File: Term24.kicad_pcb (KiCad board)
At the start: 4 copper layers, 100 x 60 mm, 55 parts, among them J1 USB_B, J11 VGA DE15, J14 Conn_01x06, J15 Conn_01x06, J3 DE9_Plug, J5 Mini-DIN-6, J6 Conn_01x08, J7 AudioJack3, SW1 SW_DIP_x02, SW11 SW_Push, SW2 SW_DIP_x02, SW3 SW_SPDT, U1 PIC24EP512GP202-I/SP, U5 LM1117T-3.3

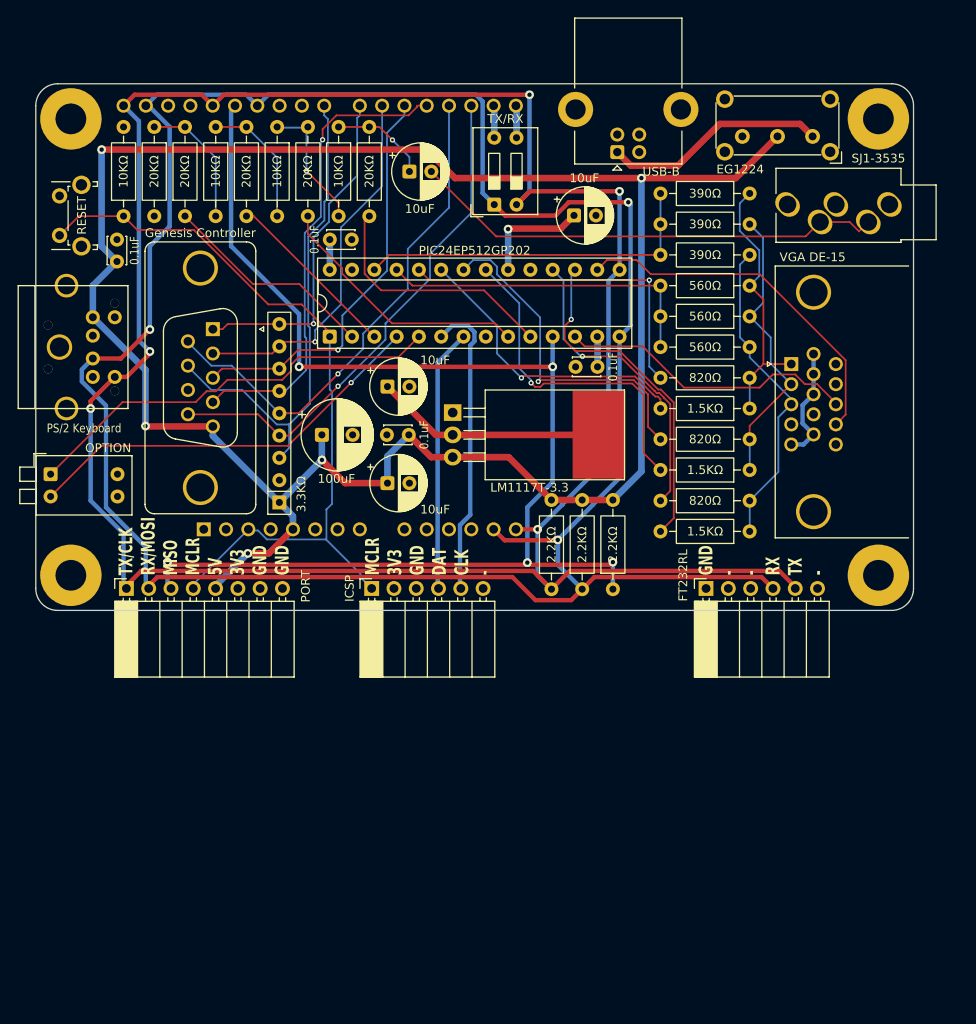
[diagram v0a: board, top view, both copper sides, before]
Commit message: Add files via upload
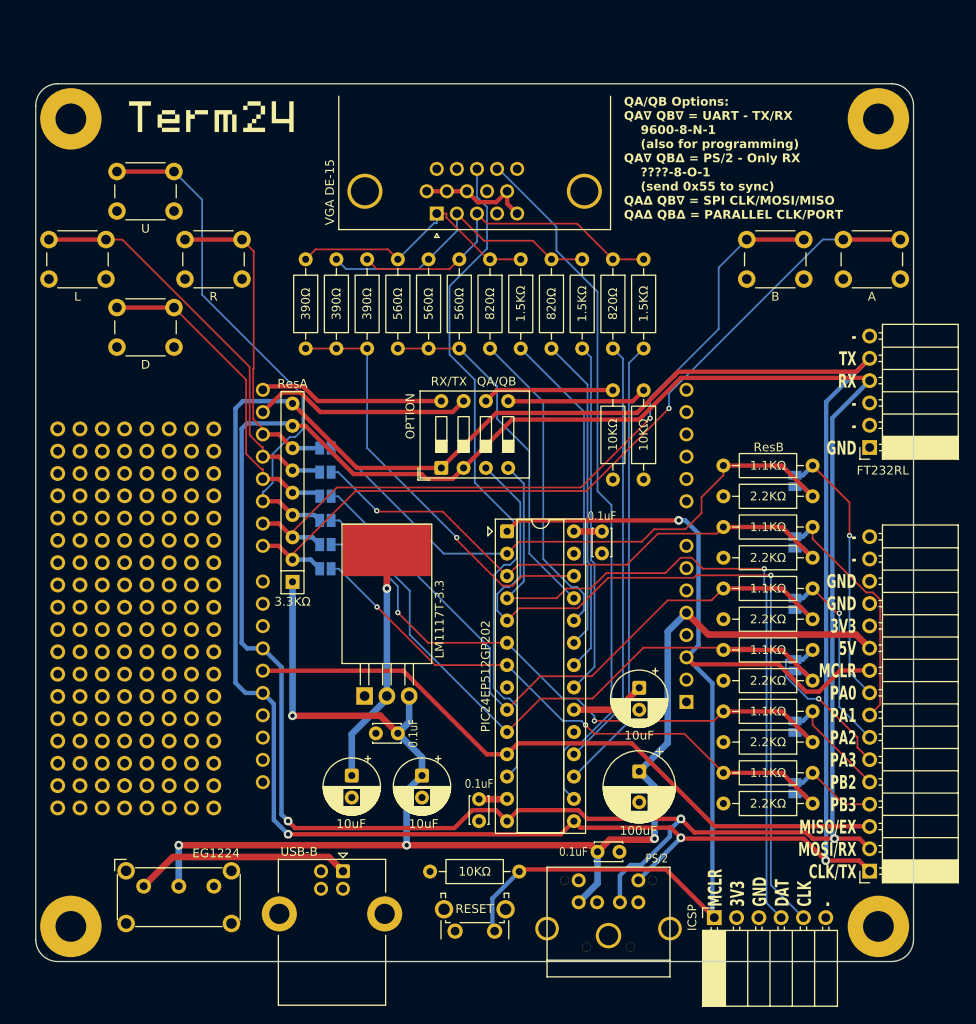
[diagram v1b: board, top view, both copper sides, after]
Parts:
- removed C24: C_Polarized_Small_US, Capacitor_THT:CP_Radial_D6.3mm_P2.50mm
- removed J3: DE9_Plug, Connector_Dsub:DSUB-9_Pins_Vertical_P2.77x2.84mm_MountingHoles
- removed J6: Conn_01x08, Connector_PinSocket_2.54mm:PinSocket_1x08_P2.54mm_Horizontal
- removed J7: AudioJack3, Connector_Audio:Jack_3.5mm_CUI_SJ1-3535NG_Horizontal_CircularHoles
- removed R21, R22, R23, R24, R25, R26, R27, R4, R5, R6: R_US, Resistor_THT:R_Axial_DIN0207_L6.3mm_D2.5mm_P10.16mm_Horizontal
- removed SW1: SW_DIP_x02, Button_Switch_THT:SW_DIP_SPSTx02_Slide_9.78x7.26mm_W7.62mm_P2.54mm
- removed SW2: SW_DIP_x02, Button_Switch_THT:SW_DIP_SPSTx02_Piano_10.8x6.64mm_W7.62mm_P2.54mm
- added J2: Conn_01x16, Connector_PinSocket_2.54mm:PinSocket_1x16_P2.54mm_Horizontal, F.Cu at (145.0, 139.7)
- added JP1: Jumper_2_Open, Jumper:SolderJumper-2_P1.3mm_Open_Pad1.0x1.5mm, B.Cu at (136.5, 95.2)
- added JP10: Jumper_2_Open, Jumper:SolderJumper-2_P1.3mm_Open_Pad1.0x1.5mm, B.Cu at (83.0, 99.8)
- added JP11: Jumper_2_Open, Jumper:SolderJumper-2_P1.3mm_Open_Pad1.0x1.5mm, B.Cu at (83.0, 102.5)
- added JP12: Jumper_2_Open, Jumper:SolderJumper-2_P1.3mm_Open_Pad1.0x1.5mm, B.Cu at (83.0, 105.2)
- added JP2: Jumper_2_Open, Jumper:SolderJumper-2_P1.3mm_Open_Pad1.0x1.5mm, B.Cu at (136.5, 102.2)
- added JP3: Jumper_2_Open, Jumper:SolderJumper-2_P1.3mm_Open_Pad1.0x1.5mm, B.Cu at (136.5, 109.2)
- added JP4: Jumper_2_Open, Jumper:SolderJumper-2_P1.3mm_Open_Pad1.0x1.5mm, B.Cu at (136.5, 116.2)
- added JP5: Jumper_2_Open, Jumper:SolderJumper-2_P1.3mm_Open_Pad1.0x1.5mm, B.Cu at (136.5, 123.2)
- added JP6: Jumper_2_Open, Jumper:SolderJumper-2_P1.3mm_Open_Pad1.0x1.5mm, B.Cu at (136.5, 130.2)
- added JP7: Jumper_2_Open, Jumper:SolderJumper-2_P1.3mm_Open_Pad1.0x1.5mm, B.Cu at (83.0, 91.5)
- added JP8: Jumper_2_Open, Jumper:SolderJumper-2_P1.3mm_Open_Pad1.0x1.5mm, B.Cu at (83.0, 94.2)
- added JP9: Jumper_2_Open, Jumper:SolderJumper-2_P1.3mm_Open_Pad1.0x1.5mm, B.Cu at (83.0, 97.0)
- added R33: R_US, Resistor_THT:R_Axial_DIN0207_L6.3mm_D2.5mm_P10.16mm_Horizontal, F.Cu at (115.8, 95.1)
- added R34: R_US, Resistor_THT:R_Axial_DIN0207_L6.3mm_D2.5mm_P10.16mm_Horizontal, F.Cu at (119.2, 95.1)
- added R35: R_US, Resistor_THT:R_Axial_DIN0207_L6.3mm_D2.5mm_P10.16mm_Horizontal, F.Cu at (138.5, 93.5)
- added R37: R_US, Resistor_THT:R_Axial_DIN0207_L6.3mm_D2.5mm_P10.16mm_Horizontal, F.Cu at (138.5, 100.5)
- added R38: R_US, Resistor_THT:R_Axial_DIN0207_L6.3mm_D2.5mm_P10.16mm_Horizontal, F.Cu at (138.5, 104.0)
- added R39: R_US, Resistor_THT:R_Axial_DIN0207_L6.3mm_D2.5mm_P10.16mm_Horizontal, F.Cu at (138.5, 107.5)
- added R40: R_US, Resistor_THT:R_Axial_DIN0207_L6.3mm_D2.5mm_P10.16mm_Horizontal, F.Cu at (138.5, 111.0)
- added R41: R_US, Resistor_THT:R_Axial_DIN0207_L6.3mm_D2.5mm_P10.16mm_Horizontal, F.Cu at (138.5, 114.5)
- added R42: R_US, Resistor_THT:R_Axial_DIN0207_L6.3mm_D2.5mm_P10.16mm_Horizontal, F.Cu at (138.5, 118.0)
- added R43: R_US, Resistor_THT:R_Axial_DIN0207_L6.3mm_D2.5mm_P10.16mm_Horizontal, F.Cu at (138.5, 121.5)
- added R44: R_US, Resistor_THT:R_Axial_DIN0207_L6.3mm_D2.5mm_P10.16mm_Horizontal, F.Cu at (138.5, 125.0)
- added R45: R_US, Resistor_THT:R_Axial_DIN0207_L6.3mm_D2.5mm_P10.16mm_Horizontal, F.Cu at (138.5, 128.5)
- added R46: R_US, Resistor_THT:R_Axial_DIN0207_L6.3mm_D2.5mm_P10.16mm_Horizontal, F.Cu at (138.5, 132.0)
- added SW10: SW_DIP_x04, Button_Switch_THT:SW_DIP_SPSTx04_Slide_9.78x12.34mm_W7.62mm_P2.54mm, F.Cu at (96.2, 93.8)
- added SW4: SW_Push, Button_Switch_THT:SW_PUSH_6mm_H7.3mm, F.Cu at (59.2, 60.0)
- added SW5: SW_Push, Button_Switch_THT:SW_PUSH_6mm_H7.3mm, F.Cu at (59.2, 75.5)
- added SW6: SW_Push, Button_Switch_THT:SW_PUSH_6mm_H7.3mm, F.Cu at (51.5, 67.8)
- added SW7: SW_Push, Button_Switch_THT:SW_PUSH_6mm_H7.3mm, F.Cu at (67.0, 67.8)
- added SW8: SW_Push, Button_Switch_THT:SW_PUSH_6mm_H7.3mm, F.Cu at (142.0, 67.8)
- added SW9: SW_Push, Button_Switch_THT:SW_PUSH_6mm_H7.3mm, F.Cu at (131.0, 67.8)
- added TP1: TestPoint, Hardware:PinHeader_1x01_P2.54mm_Vertical_TestPoint, F.Cu at (52.5, 89.3)
- added TP10: TestPoint, Hardware:PinHeader_1x01_P2.54mm_Vertical_TestPoint, F.Cu at (67.7, 89.3)
- added TP100: TestPoint, Hardware:PinHeader_1x01_P2.54mm_Vertical_TestPoint, F.Cu at (70.3, 117.3)
- added TP101: TestPoint, Hardware:PinHeader_1x01_P2.54mm_Vertical_TestPoint, F.Cu at (52.5, 119.8)
- added TP102: TestPoint, Hardware:PinHeader_1x01_P2.54mm_Vertical_TestPoint, F.Cu at (52.5, 122.3)
- added TP103: TestPoint, Hardware:PinHeader_1x01_P2.54mm_Vertical_TestPoint, F.Cu at (52.5, 124.9)
- added TP104: TestPoint, Hardware:PinHeader_1x01_P2.54mm_Vertical_TestPoint, F.Cu at (52.5, 127.4)
- added TP105: TestPoint, Hardware:PinHeader_1x01_P2.54mm_Vertical_TestPoint, F.Cu at (52.5, 130.0)
- added TP106: TestPoint, Hardware:PinHeader_1x01_P2.54mm_Vertical_TestPoint, F.Cu at (52.5, 132.5)
- added TP107: TestPoint, Hardware:PinHeader_1x01_P2.54mm_Vertical_TestPoint, F.Cu at (55.0, 119.8)
- added TP108: TestPoint, Hardware:PinHeader_1x01_P2.54mm_Vertical_TestPoint, F.Cu at (55.0, 122.3)
- added TP109: TestPoint, Hardware:PinHeader_1x01_P2.54mm_Vertical_TestPoint, F.Cu at (55.0, 124.9)
- added TP11: TestPoint, Hardware:PinHeader_1x01_P2.54mm_Vertical_TestPoint, F.Cu at (60.1, 89.3)
- added TP110: TestPoint, Hardware:PinHeader_1x01_P2.54mm_Vertical_TestPoint, F.Cu at (55.0, 127.4)
- added TP111: TestPoint, Hardware:PinHeader_1x01_P2.54mm_Vertical_TestPoint, F.Cu at (55.0, 130.0)
- added TP112: TestPoint, Hardware:PinHeader_1x01_P2.54mm_Vertical_TestPoint, F.Cu at (55.0, 132.5)
- added TP113: TestPoint, Hardware:PinHeader_1x01_P2.54mm_Vertical_TestPoint, F.Cu at (57.6, 119.8)
- added TP114: TestPoint, Hardware:PinHeader_1x01_P2.54mm_Vertical_TestPoint, F.Cu at (57.6, 122.3)
- added TP115: TestPoint, Hardware:PinHeader_1x01_P2.54mm_Vertical_TestPoint, F.Cu at (57.6, 124.9)
- added TP116: TestPoint, Hardware:PinHeader_1x01_P2.54mm_Vertical_TestPoint, F.Cu at (57.6, 127.4)
- added TP117: TestPoint, Hardware:PinHeader_1x01_P2.54mm_Vertical_TestPoint, F.Cu at (57.6, 130.0)
- added TP118: TestPoint, Hardware:PinHeader_1x01_P2.54mm_Vertical_TestPoint, F.Cu at (57.6, 132.5)
- added TP119: TestPoint, Hardware:PinHeader_1x01_P2.54mm_Vertical_TestPoint, F.Cu at (60.1, 119.8)
- added TP12: TestPoint, Hardware:PinHeader_1x01_P2.54mm_Vertical_TestPoint, F.Cu at (70.3, 89.3)
- added TP120: TestPoint, Hardware:PinHeader_1x01_P2.54mm_Vertical_TestPoint, F.Cu at (60.1, 122.3)
- added TP121: TestPoint, Hardware:PinHeader_1x01_P2.54mm_Vertical_TestPoint, F.Cu at (60.1, 124.9)
- added TP122: TestPoint, Hardware:PinHeader_1x01_P2.54mm_Vertical_TestPoint, F.Cu at (60.1, 127.4)
- added TP123: TestPoint, Hardware:PinHeader_1x01_P2.54mm_Vertical_TestPoint, F.Cu at (60.1, 130.0)
- added TP124: TestPoint, Hardware:PinHeader_1x01_P2.54mm_Vertical_TestPoint, F.Cu at (60.1, 132.5)
- added TP125: TestPoint, Hardware:PinHeader_1x01_P2.54mm_Vertical_TestPoint, F.Cu at (62.7, 119.8)
- added TP126: TestPoint, Hardware:PinHeader_1x01_P2.54mm_Vertical_TestPoint, F.Cu at (62.7, 122.3)
- added TP127: TestPoint, Hardware:PinHeader_1x01_P2.54mm_Vertical_TestPoint, F.Cu at (62.7, 124.9)
- added TP128: TestPoint, Hardware:PinHeader_1x01_P2.54mm_Vertical_TestPoint, F.Cu at (62.7, 127.4)
- added TP129: TestPoint, Hardware:PinHeader_1x01_P2.54mm_Vertical_TestPoint, F.Cu at (62.7, 130.0)
- added TP13: TestPoint, Hardware:PinHeader_1x01_P2.54mm_Vertical_TestPoint, F.Cu at (52.5, 91.9)
- added TP130: TestPoint, Hardware:PinHeader_1x01_P2.54mm_Vertical_TestPoint, F.Cu at (62.7, 132.5)
- added TP131: TestPoint, Hardware:PinHeader_1x01_P2.54mm_Vertical_TestPoint, F.Cu at (65.2, 119.8)
- added TP132: TestPoint, Hardware:PinHeader_1x01_P2.54mm_Vertical_TestPoint, F.Cu at (65.2, 122.3)
- added TP133: TestPoint, Hardware:PinHeader_1x01_P2.54mm_Vertical_TestPoint, F.Cu at (65.2, 124.9)
- added TP134: TestPoint, Hardware:PinHeader_1x01_P2.54mm_Vertical_TestPoint, F.Cu at (65.2, 127.4)
- added TP135: TestPoint, Hardware:PinHeader_1x01_P2.54mm_Vertical_TestPoint, F.Cu at (65.2, 130.0)
- added TP136: TestPoint, Hardware:PinHeader_1x01_P2.54mm_Vertical_TestPoint, F.Cu at (65.2, 132.5)
- added TP137: TestPoint, Hardware:PinHeader_1x01_P2.54mm_Vertical_TestPoint, F.Cu at (67.7, 119.8)
- added TP138: TestPoint, Hardware:PinHeader_1x01_P2.54mm_Vertical_TestPoint, F.Cu at (67.7, 122.3)
- added TP139: TestPoint, Hardware:PinHeader_1x01_P2.54mm_Vertical_TestPoint, F.Cu at (67.7, 124.9)
- added TP14: TestPoint, Hardware:PinHeader_1x01_P2.54mm_Vertical_TestPoint, F.Cu at (55.0, 91.9)
- added TP140: TestPoint, Hardware:PinHeader_1x01_P2.54mm_Vertical_TestPoint, F.Cu at (67.7, 127.4)
- added TP141: TestPoint, Hardware:PinHeader_1x01_P2.54mm_Vertical_TestPoint, F.Cu at (67.7, 130.0)
- added TP142: TestPoint, Hardware:PinHeader_1x01_P2.54mm_Vertical_TestPoint, F.Cu at (67.7, 132.5)
- added TP143: TestPoint, Hardware:PinHeader_1x01_P2.54mm_Vertical_TestPoint, F.Cu at (70.3, 119.8)
- added TP144: TestPoint, Hardware:PinHeader_1x01_P2.54mm_Vertical_TestPoint, F.Cu at (70.3, 122.3)
- added TP145: TestPoint, Hardware:PinHeader_1x01_P2.54mm_Vertical_TestPoint, F.Cu at (70.3, 124.9)
- added TP146: TestPoint, Hardware:PinHeader_1x01_P2.54mm_Vertical_TestPoint, F.Cu at (70.3, 127.4)
- added TP147: TestPoint, Hardware:PinHeader_1x01_P2.54mm_Vertical_TestPoint, F.Cu at (70.3, 130.0)
- added TP148: TestPoint, Hardware:PinHeader_1x01_P2.54mm_Vertical_TestPoint, F.Cu at (70.3, 132.5)
- added TP15: TestPoint, Hardware:PinHeader_1x01_P2.54mm_Vertical_TestPoint, F.Cu at (55.0, 94.4)
- added TP16: TestPoint, Hardware:PinHeader_1x01_P2.54mm_Vertical_TestPoint, F.Cu at (52.5, 99.5)
- added TP17: TestPoint, Hardware:PinHeader_1x01_P2.54mm_Vertical_TestPoint, F.Cu at (52.5, 102.0)
- added TP18: TestPoint, Hardware:PinHeader_1x01_P2.54mm_Vertical_TestPoint, F.Cu at (52.5, 104.6)
- added TP19: TestPoint, Hardware:PinHeader_1x01_P2.54mm_Vertical_TestPoint, F.Cu at (52.5, 107.1)
- added TP20: TestPoint, Hardware:PinHeader_1x01_P2.54mm_Vertical_TestPoint, F.Cu at (52.5, 109.6)
- added TP21: TestPoint, Hardware:PinHeader_1x01_P2.54mm_Vertical_TestPoint, F.Cu at (52.5, 112.2)
- added TP22: TestPoint, Hardware:PinHeader_1x01_P2.54mm_Vertical_TestPoint, F.Cu at (52.5, 114.7)
- added TP23: TestPoint, Hardware:PinHeader_1x01_P2.54mm_Vertical_TestPoint, F.Cu at (52.5, 117.3)
- added TP24: TestPoint, Hardware:PinHeader_1x01_P2.54mm_Vertical_TestPoint, F.Cu at (57.6, 91.9)
- added TP25: TestPoint, Hardware:PinHeader_1x01_P2.54mm_Vertical_TestPoint, F.Cu at (52.5, 94.4)
- added TP26: TestPoint, Hardware:PinHeader_1x01_P2.54mm_Vertical_TestPoint, F.Cu at (57.6, 94.4)
- added TP27: TestPoint, Hardware:PinHeader_1x01_P2.54mm_Vertical_TestPoint, F.Cu at (55.0, 99.5)
- added TP28: TestPoint, Hardware:PinHeader_1x01_P2.54mm_Vertical_TestPoint, F.Cu at (55.0, 102.0)
- added TP29: TestPoint, Hardware:PinHeader_1x01_P2.54mm_Vertical_TestPoint, F.Cu at (55.0, 104.6)
- added TP30: TestPoint, Hardware:PinHeader_1x01_P2.54mm_Vertical_TestPoint, F.Cu at (55.0, 107.1)
- added TP31: TestPoint, Hardware:PinHeader_1x01_P2.54mm_Vertical_TestPoint, F.Cu at (55.0, 109.6)
- added TP32: TestPoint, Hardware:PinHeader_1x01_P2.54mm_Vertical_TestPoint, F.Cu at (55.0, 112.2)
- added TP33: TestPoint, Hardware:PinHeader_1x01_P2.54mm_Vertical_TestPoint, F.Cu at (55.0, 114.7)
- added TP34: TestPoint, Hardware:PinHeader_1x01_P2.54mm_Vertical_TestPoint, F.Cu at (55.0, 117.3)
- added TP35: TestPoint, Hardware:PinHeader_1x01_P2.54mm_Vertical_TestPoint, F.Cu at (60.1, 91.9)
- added TP36: TestPoint, Hardware:PinHeader_1x01_P2.54mm_Vertical_TestPoint, F.Cu at (60.1, 94.4)
- added TP37: TestPoint, Hardware:PinHeader_1x01_P2.54mm_Vertical_TestPoint, F.Cu at (52.5, 96.9)
- added TP38: TestPoint, Hardware:PinHeader_1x01_P2.54mm_Vertical_TestPoint, F.Cu at (57.6, 99.5)
- added TP39: TestPoint, Hardware:PinHeader_1x01_P2.54mm_Vertical_TestPoint, F.Cu at (57.6, 102.0)
- added TP40: TestPoint, Hardware:PinHeader_1x01_P2.54mm_Vertical_TestPoint, F.Cu at (57.6, 104.6)
- added TP41: TestPoint, Hardware:PinHeader_1x01_P2.54mm_Vertical_TestPoint, F.Cu at (57.6, 107.1)
- added TP42: TestPoint, Hardware:PinHeader_1x01_P2.54mm_Vertical_TestPoint, F.Cu at (57.6, 109.6)
- added TP43: TestPoint, Hardware:PinHeader_1x01_P2.54mm_Vertical_TestPoint, F.Cu at (57.6, 112.2)
- added TP44: TestPoint, Hardware:PinHeader_1x01_P2.54mm_Vertical_TestPoint, F.Cu at (57.6, 114.7)
- added TP45: TestPoint, Hardware:PinHeader_1x01_P2.54mm_Vertical_TestPoint, F.Cu at (57.6, 117.3)
- added TP46: TestPoint, Hardware:PinHeader_1x01_P2.54mm_Vertical_TestPoint, F.Cu at (62.7, 91.9)
- added TP47: TestPoint, Hardware:PinHeader_1x01_P2.54mm_Vertical_TestPoint, F.Cu at (62.7, 94.4)
- added TP48: TestPoint, Hardware:PinHeader_1x01_P2.54mm_Vertical_TestPoint, F.Cu at (55.0, 96.9)
- added TP49: TestPoint, Hardware:PinHeader_1x01_P2.54mm_Vertical_TestPoint, F.Cu at (60.1, 99.5)
- added TP50: TestPoint, Hardware:PinHeader_1x01_P2.54mm_Vertical_TestPoint, F.Cu at (60.1, 102.0)
- added TP51: TestPoint, Hardware:PinHeader_1x01_P2.54mm_Vertical_TestPoint, F.Cu at (60.1, 104.6)
- added TP52: TestPoint, Hardware:PinHeader_1x01_P2.54mm_Vertical_TestPoint, F.Cu at (60.1, 107.1)
- added TP53: TestPoint, Hardware:PinHeader_1x01_P2.54mm_Vertical_TestPoint, F.Cu at (60.1, 109.6)
- added TP54: TestPoint, Hardware:PinHeader_1x01_P2.54mm_Vertical_TestPoint, F.Cu at (60.1, 112.2)
- added TP55: TestPoint, Hardware:PinHeader_1x01_P2.54mm_Vertical_TestPoint, F.Cu at (60.1, 114.7)
- added TP56: TestPoint, Hardware:PinHeader_1x01_P2.54mm_Vertical_TestPoint, F.Cu at (60.1, 117.3)
- added TP57: TestPoint, Hardware:PinHeader_1x01_P2.54mm_Vertical_TestPoint, F.Cu at (65.2, 91.9)
- added TP58: TestPoint, Hardware:PinHeader_1x01_P2.54mm_Vertical_TestPoint, F.Cu at (65.2, 94.4)
- added TP59: TestPoint, Hardware:PinHeader_1x01_P2.54mm_Vertical_TestPoint, F.Cu at (57.6, 96.9)
- added TP6: TestPoint, Hardware:PinHeader_1x01_P2.54mm_Vertical_TestPoint, F.Cu at (62.7, 89.3)
- added TP60: TestPoint, Hardware:PinHeader_1x01_P2.54mm_Vertical_TestPoint, F.Cu at (62.7, 99.5)
- added TP61: TestPoint, Hardware:PinHeader_1x01_P2.54mm_Vertical_TestPoint, F.Cu at (62.7, 102.0)
- added TP62: TestPoint, Hardware:PinHeader_1x01_P2.54mm_Vertical_TestPoint, F.Cu at (62.7, 104.6)
- added TP63: TestPoint, Hardware:PinHeader_1x01_P2.54mm_Vertical_TestPoint, F.Cu at (62.7, 107.1)
- added TP64: TestPoint, Hardware:PinHeader_1x01_P2.54mm_Vertical_TestPoint, F.Cu at (62.7, 109.6)
- added TP65: TestPoint, Hardware:PinHeader_1x01_P2.54mm_Vertical_TestPoint, F.Cu at (62.7, 112.2)
- added TP66: TestPoint, Hardware:PinHeader_1x01_P2.54mm_Vertical_TestPoint, F.Cu at (62.7, 114.7)
- added TP67: TestPoint, Hardware:PinHeader_1x01_P2.54mm_Vertical_TestPoint, F.Cu at (62.7, 117.3)
- added TP68: TestPoint, Hardware:PinHeader_1x01_P2.54mm_Vertical_TestPoint, F.Cu at (67.7, 91.9)
- added TP69: TestPoint, Hardware:PinHeader_1x01_P2.54mm_Vertical_TestPoint, F.Cu at (67.7, 94.4)
- added TP7: TestPoint, Hardware:PinHeader_1x01_P2.54mm_Vertical_TestPoint, F.Cu at (55.0, 89.3)
- added TP70: TestPoint, Hardware:PinHeader_1x01_P2.54mm_Vertical_TestPoint, F.Cu at (60.1, 96.9)
- added TP71: TestPoint, Hardware:PinHeader_1x01_P2.54mm_Vertical_TestPoint, F.Cu at (65.2, 99.5)
- added TP72: TestPoint, Hardware:PinHeader_1x01_P2.54mm_Vertical_TestPoint, F.Cu at (65.2, 102.0)
- added TP73: TestPoint, Hardware:PinHeader_1x01_P2.54mm_Vertical_TestPoint, F.Cu at (65.2, 104.6)
- added TP74: TestPoint, Hardware:PinHeader_1x01_P2.54mm_Vertical_TestPoint, F.Cu at (65.2, 107.1)
- added TP75: TestPoint, Hardware:PinHeader_1x01_P2.54mm_Vertical_TestPoint, F.Cu at (65.2, 109.6)
- added TP76: TestPoint, Hardware:PinHeader_1x01_P2.54mm_Vertical_TestPoint, F.Cu at (65.2, 112.2)
- added TP77: TestPoint, Hardware:PinHeader_1x01_P2.54mm_Vertical_TestPoint, F.Cu at (65.2, 114.7)
- added TP78: TestPoint, Hardware:PinHeader_1x01_P2.54mm_Vertical_TestPoint, F.Cu at (65.2, 117.3)
- added TP79: TestPoint, Hardware:PinHeader_1x01_P2.54mm_Vertical_TestPoint, F.Cu at (70.3, 91.9)
- added TP8: TestPoint, Hardware:PinHeader_1x01_P2.54mm_Vertical_TestPoint, F.Cu at (65.2, 89.3)
- added TP80: TestPoint, Hardware:PinHeader_1x01_P2.54mm_Vertical_TestPoint, F.Cu at (67.7, 96.9)
- added TP81: TestPoint, Hardware:PinHeader_1x01_P2.54mm_Vertical_TestPoint, F.Cu at (62.7, 96.9)
- added TP82: TestPoint, Hardware:PinHeader_1x01_P2.54mm_Vertical_TestPoint, F.Cu at (67.7, 99.5)
- added TP83: TestPoint, Hardware:PinHeader_1x01_P2.54mm_Vertical_TestPoint, F.Cu at (67.7, 102.0)
- added TP84: TestPoint, Hardware:PinHeader_1x01_P2.54mm_Vertical_TestPoint, F.Cu at (67.7, 104.6)
- added TP85: TestPoint, Hardware:PinHeader_1x01_P2.54mm_Vertical_TestPoint, F.Cu at (67.7, 107.1)
- added TP86: TestPoint, Hardware:PinHeader_1x01_P2.54mm_Vertical_TestPoint, F.Cu at (67.7, 109.6)
- added TP87: TestPoint, Hardware:PinHeader_1x01_P2.54mm_Vertical_TestPoint, F.Cu at (67.7, 112.2)
- added TP88: TestPoint, Hardware:PinHeader_1x01_P2.54mm_Vertical_TestPoint, F.Cu at (67.7, 114.7)
- added TP89: TestPoint, Hardware:PinHeader_1x01_P2.54mm_Vertical_TestPoint, F.Cu at (67.7, 117.3)
- added TP9: TestPoint, Hardware:PinHeader_1x01_P2.54mm_Vertical_TestPoint, F.Cu at (57.6, 89.3)
- added TP90: TestPoint, Hardware:PinHeader_1x01_P2.54mm_Vertical_TestPoint, F.Cu at (70.3, 94.4)
- added TP91: TestPoint, Hardware:PinHeader_1x01_P2.54mm_Vertical_TestPoint, F.Cu at (70.3, 96.9)
- added TP92: TestPoint, Hardware:PinHeader_1x01_P2.54mm_Vertical_TestPoint, F.Cu at (65.2, 96.9)
- added TP93: TestPoint, Hardware:PinHeader_1x01_P2.54mm_Vertical_TestPoint, F.Cu at (70.3, 99.5)
- added TP94: TestPoint, Hardware:PinHeader_1x01_P2.54mm_Vertical_TestPoint, F.Cu at (70.3, 102.0)
- added TP95: TestPoint, Hardware:PinHeader_1x01_P2.54mm_Vertical_TestPoint, F.Cu at (70.3, 104.6)
- added TP96: TestPoint, Hardware:PinHeader_1x01_P2.54mm_Vertical_TestPoint, F.Cu at (70.3, 107.1)
- added TP97: TestPoint, Hardware:PinHeader_1x01_P2.54mm_Vertical_TestPoint, F.Cu at (70.3, 109.6)
- added TP98: TestPoint, Hardware:PinHeader_1x01_P2.54mm_Vertical_TestPoint, F.Cu at (70.3, 112.2)
- added TP99: TestPoint, Hardware:PinHeader_1x01_P2.54mm_Vertical_TestPoint, F.Cu at (70.3, 114.7)
- G102: moved to F.Cu
- moved SW3 114.5 mm to (62.3, 141.4), turned to 0 degrees
- moved SW11 93.5 mm to (102.3, 146.5), turned to 180 degrees
- moved C26 90.2 mm to (116.5, 137.5), turned to 180 degrees
- moved J5 89.5 mm to (115.2, 145.5), turned to 180 degrees
- moved J1 87.7 mm to (85.0, 139.7), turned to -90 degrees
- moved R2 87.2 mm to (105.1, 139.8), turned to 180 degrees
- moved R36 86.0 mm to (138.5, 97.0), turned to 180 degrees
- moved G101 70.7 mm to (87.8, 54.2), turned to 180 degrees
- moved A1 58.4 mm to (124.1, 120.4), turned to 90 degrees
- moved C1 54.3 mm to (118.8, 118.8), turned to -90 degrees
- moved J14 54.1 mm to (127.3, 145.0)
- moved C19 52.9 mm to (100.5, 134.0), turned to 90 degrees
- moved C2 52.7 mm to (118.8, 128.3), turned to -90 degrees
- moved R30 51.1 mm to (80.8, 70.0), turned to -90 degrees
- moved R31 47.2 mm to (84.2, 70.0), turned to -90 degrees
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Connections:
- net SERIAL-MISO renamed SERIAL-MISO-EX
- A1 pad 13: SERIAL-MOSI-RX-SDA -> unconnected-(A1-SDA/A4-Pad13)
- A1 pad 14: SERIAL-CLK-TX-SCL -> unconnected-(A1-SCL/A5-Pad14)
- A1 pad 15: Net-(A1-D0/RX) -> UNO-RX
- A1 pad 16: Net-(A1-D1/TX) -> UNO-TX
- A1 pad 17: JOY-BUTTON2 -> JOY-R
- A1 pad 18: JOY-BUTTON1 -> JOY-L
- A1 pad 19: JOY-RIGHT -> JOY-D
- A1 pad 20: JOY-LEFT -> JOY-U
- A1 pad 21: JOY-DOWN -> JOY-B
- A1 pad 22: JOY-UP -> JOY-A
- A1 pad 23: JOY-SELECT -> unconnected-(A1-D8-Pad23)
- A1 pad 26: SERIAL-MOSI-RX-SDA -> SERIAL-MOSI-RX
- A1 pad 28: SERIAL-CLK-TX-SCL -> SERIAL-CLK-TX
- A1 pad 31: SERIAL-MOSI-RX-SDA -> unconnected-(A1-SDA/A4-Pad31)
- A1 pad 32: SERIAL-CLK-TX-SCL -> unconnected-(A1-SCL/A5-Pad32)
- J15 pad 4: SERIAL-MOSI-RX-SDA -> SERIAL-MOSI-RX
- J15 pad 5: SERIAL-CLK-TX-SCL -> SERIAL-CLK-TX
- J5 pad 1: SERIAL-MOSI-RX-SDA -> SERIAL-MOSI-RX
- J5 pad 5: SERIAL-CLK-TX-SCL -> SERIAL-CLK-TX
- R36 pad 1: Net-(R21-Pad2) -> PORT-A0-3V3
- RN1 pad 2: unconnected-(RN1-R1-Pad2) -> JOY-A
- RN1 pad 3: JOY-SELECT -> JOY-B
- RN1 pad 4: JOY-BUTTON2 -> JOY-U
- RN1 pad 5: JOY-BUTTON1 -> JOY-D
- RN1 pad 6: JOY-RIGHT -> JOY-L
- RN1 pad 7: JOY-LEFT -> JOY-R
- RN1 pad 8: JOY-DOWN -> SERIAL-MOSI-RX
- RN1 pad 9: JOY-UP -> SERIAL-CLK-TX
- U1 pad 10: AUDIO-A -> PORT-A3-3V3
- U1 pad 14: SERIAL-MOSI-RX-SDA -> SERIAL-MOSI-RX
- U1 pad 15: SERIAL-CLK-TX-SCL -> SERIAL-CLK-TX
- U1 pad 2: AUDIO-D -> PORT-A0-3V3
- U1 pad 3: AUDIO-C -> PORT-A1-3V3
- U1 pad 4: OPTION-B -> ICSP-DAT
- U1 pad 5: OPTION-A -> ICSP-CLK
- U1 pad 6: ICSP-CLK -> PORT-B2-3V3
- U1 pad 7: ICSP-DAT -> PORT-B3-3V3
- U1 pad 9: AUDIO-B -> PORT-A2-3V3
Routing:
- net SERIAL-CLK-TX: track 0.00 -> 268.4 mm, vias 0 -> 3
- net SERIAL-CLK-TX-SCL: track 267.0 -> 0.00 mm, vias 5 -> 0
- net SERIAL-MOSI-RX-SDA: track 265.7 -> 0.00 mm, vias 3 -> 0
- net SERIAL-MOSI-RX: track 0.00 -> 264.7 mm, vias 0 -> 3
- net JOY-A: track 0.00 -> 93.1 mm, vias 0 -> 1
- net JOY-B: track 0.00 -> 85.4 mm, vias 0 -> 1
- net PORT-A3-3V3: track 0.00 -> 79.1 mm
- net PORT-A2-3V3: track 0.00 -> 77.5 mm
- net +5V: track 240.3 -> 165.2 mm, vias 5 -> 4
- net PORT-B2-3V3: track 0.00 -> 69.6 mm, vias 0 -> 2
- net PORT-A0-3V3: track 0.00 -> 69.6 mm
- net SERIAL-MISO-EX: track 146.6 -> 77.5 mm, vias 5 -> 0
- net PORT-B3-3V3: track 0.00 -> 68.4 mm, vias 0 -> 2
- net PORT-A1-3V3: track 0.00 -> 66.0 mm, vias 0 -> 1
- net JOY-U: track 0.00 -> 59.8 mm
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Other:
- board size 100 x 60 mm -> 100 x 100 mm
- board text added: "- - GND GND 3V3 5V MCLR PA0 PA1 PA2 PA3 PB2 PB3 MISO/EX MOSI/RX CLK/TX"
- board text added: "- TX RX - - GND"
- board text added: "3V3 Tolerant Port? (Remove ResB)"
- board text added: "Buttons to Port? (Remove ResA)"
- board text added: "OPTION"
- board text added: "Professor Steven Chad Burrow stevenchadburrow@gmail.com github.com/stevenchadburrow youtube.com/user/stevenchadburrow July 2026"
- board text added: "QA/QB"
- board text added: "QA/QB Options: QA∇ QB∇ = UART - TX/RX 9600-8-N-1 (also for programming) QA∇ QBΔ = PS/2 - Only RX ????-8-O-1 (send 0x55 to sync) QAΔ QB∇ = SPI CLK/MOSI/MISO QAΔ QBΔ = PARALLEL CLK/PORT"
- board text added: "RX/TX"
- board text added: "ResA"
- board text added: "ResB"
- board text removed: "GND - - RX TX -"
- board text removed: "July 2026 Professor Steven Chad Burrow stevenchadburrow@gmail.com youtube.com/user/stevenchadburrow github.com/stevenchadburrow"
- board text removed: "TX/CLK RX/MOSI MISO MCLR 5V 3V3 GND GND"
